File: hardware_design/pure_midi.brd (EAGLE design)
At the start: 68.8 x 100 mm, 79 parts, among them IC1 74HCT125D, IC1_33 VOLTAGE_REG_POSDT, IC2 VOLTAGE_REG_POS05DT, IC3 74HC148D, IC4 74HCT125D, Q1 20MHz, Q2 12MHz, T1 MMBT3904, T2 MMBT3904, T3 MMBT3904, T4 MMBT3904, U1 ANALOG_DEVICES_INC_AD5754AREZ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, U2 TEXAS_INSTRUMENTS_LM4040C25ID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, U3 ATMEGA328P_TQFP, U4 MAX3421, X1 OG-MIDI_MAB5SHCUI-SD-50BV, X2 KUSBVX

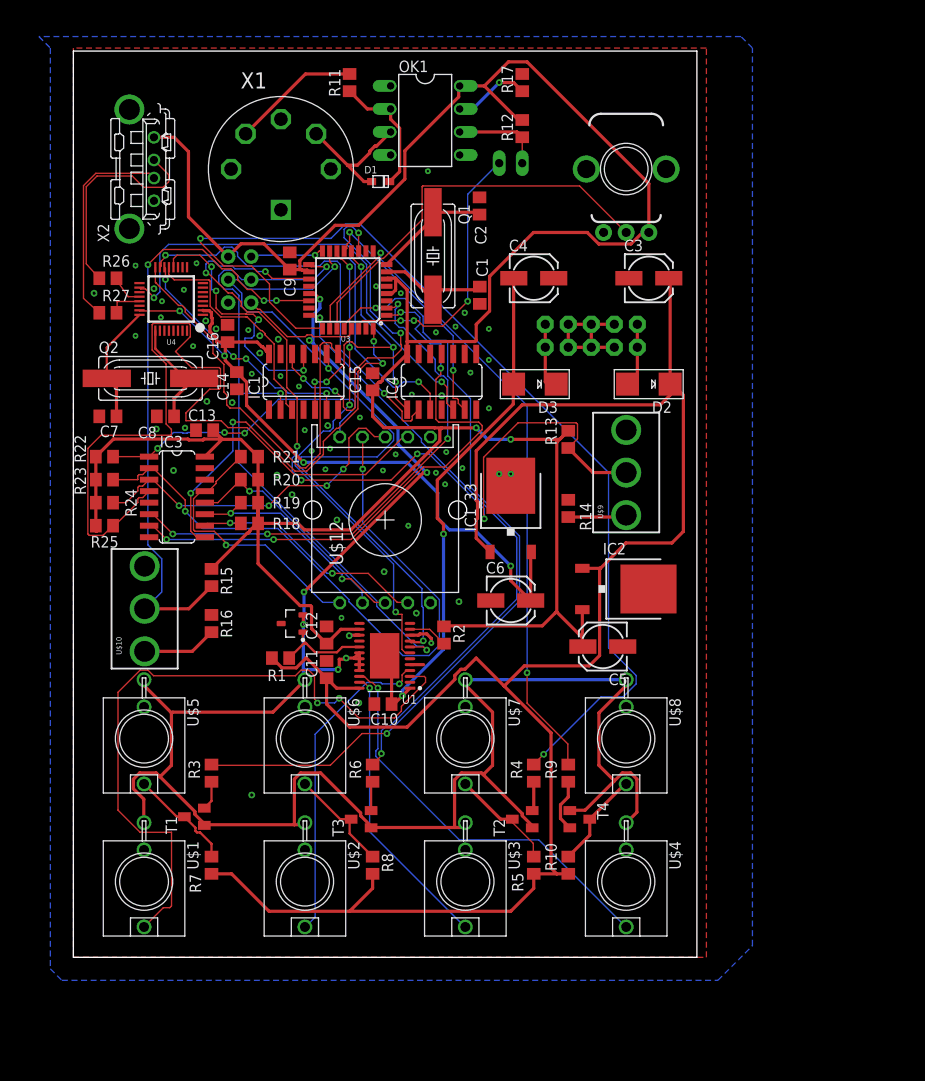
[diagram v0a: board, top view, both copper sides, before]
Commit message: Rev 1/2
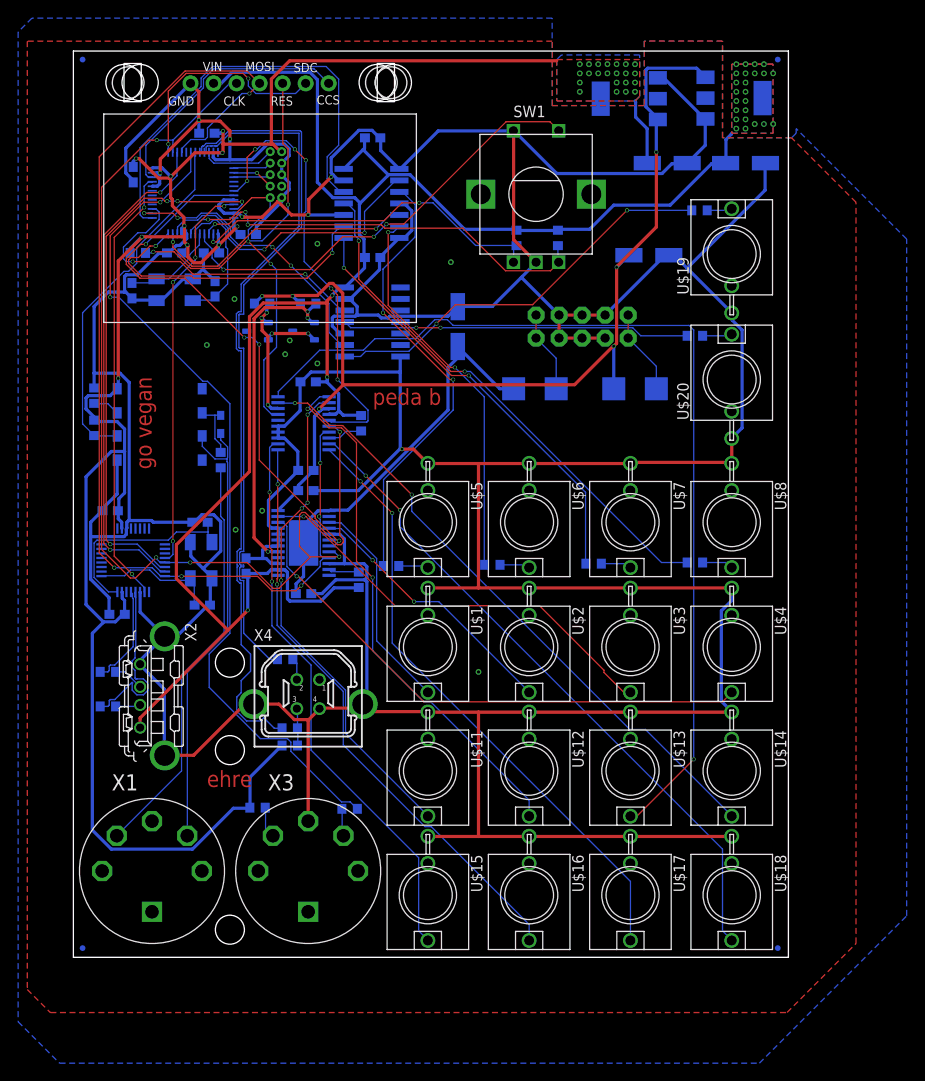
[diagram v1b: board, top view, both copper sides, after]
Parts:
- removed IC1_33: VOLTAGE_REG_POSDT, GMSN:TO252
- removed ISP1: AVRISP-6, adafruit:AVRISP
- removed JP1: (no value), jumper:JP1
- removed OK1: 6N138, optocoupler:DIL08
- removed Q1: 20MHz, adafruit:HC49UP
- removed Q2: 12MHz, adafruit:HC49UP
- removed R22, R23, R24, R25: 10k, rcl:R0805
- removed T1, T2, T3, T4: MMBT3904, transistor:SOT23-EBC
- removed U$10, U$9: TOGGLE_ON_OFF_ON, INSTRUO:TOGGLE_ON_OFF_ON
- added C17, C21, C23, C24, C25, C26: 100n, rcl:C0603
- added DI1: OLED_1.3_128X64_SPI, microbuilder:C1_ADAFRUIT_1.3_128X64_OLED
- added FD1, FD2, FD3, FD4: FIDUCIALUFIDUCIAL, SparkFun-Aesthetics:FIDUCIAL-MICRO
- added IC5: STM32F10XCXT6, stm32:TQFP48
- added IC6: LD117AS33TR, v-reg:SOT223
- added J1: CORTEX_DEBUG_PTH, SparkFun-Connectors:2X5-PTH-1.27MM
- added LOGO1: OSHW-LOGOM, SparkFun-Aesthetics:OSHW-LOGO-M
- added SW1: EC12E_SW, switch-alps:ALPS_EC12E_SW
- added U$13, U$14, U$15, U$16, U$17, U$18, U$19, U$20: WQP-PJ301M-12_JACK, thonkiconn:WQP-PJ301M-12_JACK
- added U5: TEXAS_INSTRUMENTS_LM4040C25IDBZRTEXAS_INSTRUMENTS_LM4040C25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, lm4040:TEXAS_INSTRUMENTS_LM4040C25IDBZR_1
- added X3: OG-MIDI_MAB5SHCUI-SD-50BV, yarns_v03:OG-MIDI_SD-50BV
- added X4: KUSBVX-BS1N, con-kycon:KUSBVX-BS1N
- added X6: ABRACON_ABM3B-12.000MHZ-B2-TABRACON_ABM3B-12.000MHZ-B2-T_0_0, Abracon - ABM3B-12.000MHZ-B2-T:ABRACON_ABM3B-12.000MHZ-B2-T_0
- added X7: ABRACON_ABM3B-8.000MHZ-B2-TABRACON_ABM3B-8.000MHZ-B2-T_0_0, Abracon - ABM3B-8.000MHZ-B2-T:ABRACON_ABM3B-8.000MHZ-B2-T_0
- C1, C10, C11, C12, C13, C14, C15, C16, C2, C7, C8, C9: device rcl:C0805 -> rcl:C0603
- C3, C4, C5, C6: value 47u -> 22u
- IC1: value 74HCT125D -> LD117AS50TR; device 74xx-eu:SO14 -> v-reg:SOT223
- IC2: value VOLTAGE_REG_POS05DT -> 74HCT125D; device GMSN:TO252 -> 74xx-eu:SO14
- IC3: value 74HC148D -> 6N138SMD; device 74xx-eu:SO16 -> 6n138:SO8-GW300
- R1: value 2k -> 1k; device rcl:R0805 -> rcl:R0603
- R10, R9: value 1k -> 51R; device rcl:R0805 -> rcl:R0603
- R11, R12, R17: device resistor:R0805 -> rcl:R0603
- R13, R14: value 10k -> 22R; device resistor:R0805 -> rcl:R0603
- R15, R16: device resistor:R0805 -> resistor:R0603
- R18, R19: value 10k -> 2k; device rcl:R0805 -> rcl:R0603
- R2, R21, R26, R27, R4, R5, R6, R7, R8: device rcl:R0805 -> rcl:R0603
- R20: value 10k -> 1k5; device rcl:R0805 -> rcl:R0603
- R3: value 1k -> 4k7; device rcl:R0805 -> rcl:R0603
- U$11: value Q-POT -> WQP-PJ301M-12_JACK; device INSTRUO:Q-POT -> thonkiconn:WQP-PJ301M-12_JACK
- U$12: value ALPS-SRBV -> WQP-PJ301M-12_JACK; device TomW:ALPS-SRBV -> thonkiconn:WQP-PJ301M-12_JACK
- U1: value ANALOG_DEVICES_INC_AD5754AREZANALOG_DEVICES_INC_AD5754AREZ_0_0 -> AD5676ARUZ; device Analog Devices Inc - AD5754AREZ:ANALOG_DEVICES_INC_AD5754AREZ_0 -> AD5676ARUZ:RU_20
- U2: value TEXAS_INSTRUMENTS_LM4040C25IDBZRTEXAS_INSTRUMENTS_LM4040C25IDBZR_0_1 -> AD5754BREZ; device Texas Instruments - LM4040C25IDBZR:TEXAS_INSTRUMENTS_LM4040C25IDBZR_1 -> ad5754:RE_24
- U3: value ATMEGA328P_TQFP -> TEXAS_INSTRUMENTS_LM4040C5IDBZR1; device SparkFun-IC-Microcontroller:TQFP32-08 -> lm4040:TEXAS_INSTRUMENTS_LM4040C5IDBZR_1
- moved R7 90.1 mm to (69.1, 82.4), flipped to the bottom, turned to 0 degrees
- moved X1 78.8 mm to (8.68, 9.53)
- moved U$11 69.9 mm to (39.1, 20.6), turned to 180 degrees
- moved R8 68.4 mm to (68.6, 68.6), flipped to the bottom, turned to 0 degrees
- moved C10 62.5 mm to (33.0, 90.4), flipped to the bottom, turned to 180 degrees
- moved R17 58.5 mm to (2.29, 62.0), flipped to the bottom
- moved X2 58.2 mm to (7.37, 28.8), turned to 270 degrees
- moved R12 57.6 mm to (2.29, 58.4), flipped to the bottom
- moved R16 57.2 mm to (53.5, 79.4), flipped to the bottom, turned to 90 degrees
- moved IC1 56.9 mm to (72.9, 94.8), flipped to the bottom, turned to 90 degrees
- moved C5 55.6 mm to (74.2, 87.6), flipped to the bottom, turned to 0 degrees
- moved C6 51.3 mm to (65.5, 87.6), flipped to the bottom
- moved IC2 51.0 mm to (32.9, 83.2), flipped to the bottom
- moved R15 50.4 mm to (48.9, 79.4), flipped to the bottom
- moved R26 47.2 mm to (3.81, 27.7), flipped to the bottom
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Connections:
- removed net AREF: R1.1, U1.17, U2.1
- removed net INT_USB_3V3: IC4.5, U4.18
- removed net MISO_3V3: IC4.2, U4.15
- removed net MOSI_3V3: IC1.8, U4.16
- removed net N$16: R14.2, U$9.1
- removed net N$25: C7.2, Q2.1, U4.24
- removed net N$26: IC3.11, R19.1, U$12.B
- removed net N$27: IC3.12, R20.1, U$12.C
- removed net N$28: IC3.13, R21.1, U$12.D
- removed net N$29: IC3.1, R22.1, U$12.E
- removed net N$30: IC3.2, R23.1, U$12.F
- removed net N$31: IC3.3, R24.1, U$12.G
- removed net N$32: IC3.4, R25.1, U$12.H
- removed net ROTARY_D0: IC3.9, U3.32
- removed net ROTARY_D1: IC3.7, U3.1
- removed net ROTARY_D2: IC3.6, U3.2
- removed net RST_USB_3V3: IC1.11, U4.12
- removed net SCK_3V3: IC1.3, U4.13
- removed net SPEED_VAL: U$11.P$2, U3.27
- removed net SS_DAC: U1.7, U3.14
- removed net SS_USB_3V3: IC1.6, U4.14
- removed net SWITCH0_VAL: R13.1, U$9.2, U3.19
- removed net SWITCH1_VAL: R15.1, U$10.2, U3.22
- new net AREF_25: R18.1, U2.17, U5.1
- new net AREF_5: R19.1, U1.18, U3.1
- new net CV_OUT_10: U$16.P$1, U1.11
- new net CV_OUT_11: U$17.P$1, U1.10
- new net CV_OUT_12: U$18.P$1, U1.9
- new net CV_OUT_5: U$11.P$1, U1.2
- new net CV_OUT_6: U$12.P$1, U1.1
- new net CV_OUT_7: U$13.P$1, U1.20
- new net CV_OUT_8: U$14.P$1, U1.19
- new net CV_OUT_9: U$15.P$1, U1.12
- new net D_GATE_OUT_5: IC4.9, IC5.14
- new net D_GATE_OUT_6: IC4.12, IC5.15
- new net ENC_A: IC5.2, R15.1, SW1.A
- new net ENC_B: IC5.3, R16.1, SW1.B
- new net ENC_SW: IC5.4, SW1.E
- new net GATE_OUT_5: R7.1, U$19.P$1
- new net GATE_OUT_6: R8.1, U$20.P$1
- new net JTCK: IC5.37, J1.4
- new net JTDI: IC5.38, J1.8
- new net JTDO: IC5.39, J1.6
- new net JTMS: IC5.34, J1.2
- new net MIDI_DATA_OUT: IC5.30, R9.1
- new net N$17: IC4.8, R7.2
- new net N$18: IC4.11, R8.2
- new net N$21: R13.1, X4.2
- new net N$22: R10.1, X3.4
- new net N$23: R14.1, R20.2, X4.3
- new net SDC_OLED: DI1.SDC, IC5.25
- new net SS_DAC0: IC5.42, U1.5
- new net SS_DAC1: IC5.43, U2.7
- new net SS_OLED: DI1.CCS, IC5.22
- new net USB_PER_D_N: IC5.32, R13.2
- new net USB_PER_D_P: IC5.33, R14.2
- net +12V: now also C13.1, IC1.3, IC6.3, R18.2, R19.2, U1.3, U2.24; no longer IC1_33.1, IC2.1, R1.2, R10.1, R5.1, R7.1, R8.1, U1.24
- net +3V3: now also C15.1, C21.1, C23.1, C24.1, C25.1, IC3.8, IC5.1, IC5.24, IC5.36, IC5.48, IC5.9, IC6.4, J1.1, R10.2, R12.2, R20.1, R21.2; no longer IC1.14, IC1_33.2
- net +5V: now also C10.1, C17.1, DI1.VIN, IC1.4, IC2.14, R16.2, R3.2, U1.4, U2.14; no longer C13.1, C15.1, IC2.2, IC3.16, ISP1.2, OK1.8, R12.2, R13.2, R18.2, R19.2, R20.2, R21.2, R22.2, R23.2, R24.2, R25.2, U$11.P$3, U1.14, U3.18, U3.4, U3.6
- net -12V: now also C26.2, U2.1, U2.25; no longer C10.2, U1.1, U1.25
- net CV_OUT_1: now also U2.3; no longer U1.3
- net CV_OUT_2: now also U2.4; no longer U1.4
- net CV_OUT_3: now also U2.23; no longer U1.23
- net CV_OUT_4: now also U2.22; no longer U1.22
- net D_GATE_OUT_1: now also IC2.2, IC5.10; no longer R3.2, U3.28
- net D_GATE_OUT_2: now also IC2.5, IC5.11; no longer R6.2, U3.24
- net D_GATE_OUT_3: now also IC2.9, IC5.12; no longer R4.2, U3.25
- net D_GATE_OUT_4: now also IC2.12, IC5.13; no longer R9.2, U3.26
- net GATE_OUT_1: now also R1.1; no longer R7.2, T1.C
- net GATE_OUT_2: now also R4.1; no longer R8.2, T3.C
- net GATE_OUT_3: now also R5.1; no longer R5.2, T2.C
- net GATE_OUT_4: now also R6.1; no longer R10.2, T4.C
- net GND: now also C10.2, C17.2, C21.2, C23.2, C24.2, C25.2, C26.1, DI1.GND, IC2.1, IC2.10, IC2.13, IC2.4, IC2.7, IC4.10, IC4.13, IC5.20, IC5.23, IC5.35, IC5.44, IC5.47, IC5.8, IC6.1, J1.3, J1.5, J1.9, SW1.C, SW1.D, U$11.P$3, U$12.P$3, U$13.P$3, U$14.P$3, U$15.P$3, U$16.P$3, U$17.P$3, U$18.P$3, U$19.P$3, U$20.P$3, U1.13, U1.14, U2.10, U2.15, U2.18, U2.19, U2.20, U2.21, U2.5, U3.2, U5.2, X3.2, X4.4, X4.M1, X4.M2, X6.2, X6.4, X7.2, X7.4; no longer C10.1, IC1.10, IC1.13, IC1.4, IC1.7, IC1_33.3, IC2.3, IC3.8, IC4.4, ISP1.6, OK1.5, R14.1, R16.1, T1.E, T2.E, T3.E, T4.E, U$10.3, U$11.P$1, U$12.COM, U$12.COM2, U$9.3, U1.10, U1.18, U1.19, U1.20, U1.21, U1.5, U2.2, U3.21, U3.3, U3.5
- net INT_USB: now also IC5.21, U4.18; no longer IC4.6, U3.13
- net MIDI_DATA_IN: now also IC3.6, IC5.31; no longer JP1.2, OK1.6
- net MISO: now also IC5.27, U4.15; no longer IC4.3, ISP1.1, U3.16
- net MOSI: now also DI1.MOSI, IC5.28, U1.7, U2.9, U4.16; no longer IC1.9, ISP1.4, U1.9, U3.15
- net N$1: now also U1.8; no longer U1.11
- net N$10: now also IC2.3, R1.2; no longer JP1.1, U3.30
- net N$11: now also IC2.6, R4.2; no longer R9.1, T4.B
- net N$12: now also IC3.7; no longer OK1.7
- net N$14: now also IC2.8, R5.2; no longer R16.2, U$10.1
- net N$15: now also IC2.11, R6.2; no longer IC3.10, R18.1, U$12.A
- net N$19: now also R9.2, X3.5; no longer C8.2, Q2.2, U4.25
- net N$2: now also U2.11; no longer T1.B
- net N$3: now also C2.2, IC5.6, X7.3; no longer R4.1, T2.B
- net N$4: now also IC3.2; no longer OK1.2
- net N$6: now also IC5.5, X7.1; no longer Q1.2, U3.7
- net N$7: now also C8.2, U4.25, X6.1; no longer C2.2, Q1.1, U3.8
- net N$8: now also C7.2, U4.24, X6.3; no longer R6.1, T3.B
- net N$9: now also IC3.3; no longer OK1.3
- net RST: now also DI1.RES, IC5.7, J1.10, R21.1, U1.17; no longer ISP1.5, U3.29
- net RST_USB: now also IC5.45, U4.12; no longer IC1.12, U3.11
- net SCK: now also DI1.CLK, IC5.26, U1.6, U2.8, U4.13; no longer IC1.2, ISP1.3, U1.8, U3.17
- net SS_USB: now also IC5.46, U4.14; no longer IC1.5, IC4.1, U3.12
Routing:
- net GND: track 245.0 -> 738.1 mm, vias 68 -> 19
- net +3V3: track 78.9 -> 223.1 mm, vias 4 -> 32
- net +5V: track 314.9 -> 207.4 mm, vias 2 -> 27
- net CV_OUT_7: track 0.00 -> 107.2 mm, vias 0 -> 1
- net SWITCH0_VAL: track 96.5 -> 0.00 mm, vias 6 -> 0
- net MIDI_DATA_OUT: track 0.00 -> 93.6 mm, vias 0 -> 2
- net +12V: track 212.4 -> 118.8 mm, vias 0 -> 6
- net N$32: track 91.7 -> 0.00 mm
- net USB_PER_D_P: track 0.00 -> 86.7 mm
- net D_GATE_OUT_3: track 115.7 -> 33.9 mm
- net USB_PER_D_N: track 0.00 -> 77.9 mm
- net CV_OUT_12: track 0.00 -> 73.5 mm, vias 0 -> 2
- net N$30: track 73.1 -> 0.00 mm, vias 2 -> 0
- net CV_OUT_8: track 0.00 -> 70.1 mm, vias 0 -> 2
- net SWITCH1_VAL: track 68.9 -> 0.00 mm, vias 3 -> 0
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- added copper zone on layer 1, net +3V3
- added copper zone on layer 16, net +3V3
- added copper zone on layer 1, net +5V
- added copper zone on layer 16, net +5V
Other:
- board size 68.8 x 100 mm -> 78.9 x 100 mm
- board text added: "Pure MIDI v1"
- board text added: "ehre"
- board text added: "go vegan"
- board text added: "jhbruhn 2019"
- board text added: "peda b"
- board text removed: "Pure MIDI v0.1"
- board text removed: "jhbruhn 2018"
